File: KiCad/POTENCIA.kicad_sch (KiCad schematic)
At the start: 15 parts, among them J3 Conn_01x02_Pin, J7 Conn_01x02_Pin, J8 Conn_01x02_Pin, SW7 SW_SPST, U2 LM2596S-5, U3 L298N, U7 LM1117DT-3.3

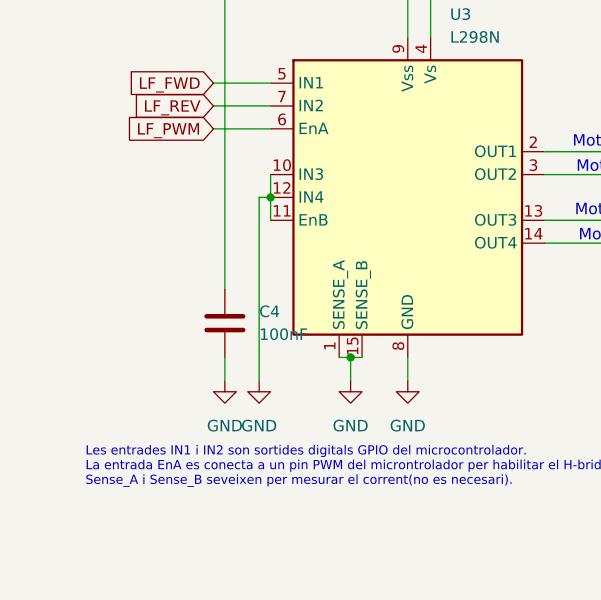
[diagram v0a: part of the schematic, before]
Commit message: aa
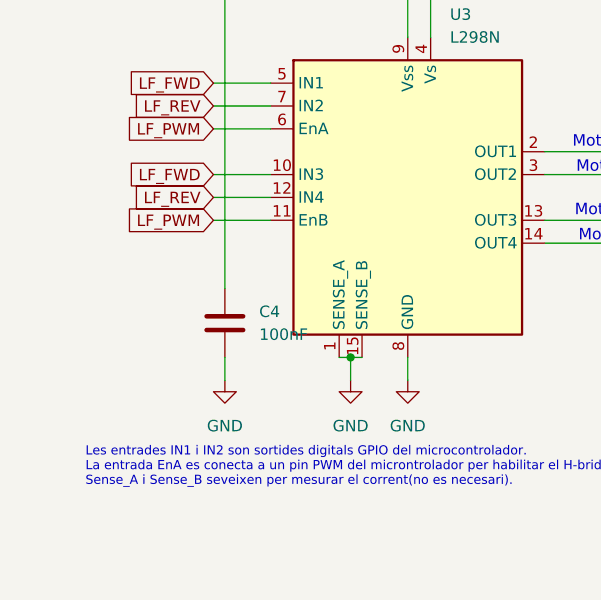
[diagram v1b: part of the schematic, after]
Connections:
- net GND: no longer U3.10 (IN3), U3.11 (EnB), U3.12 (IN4)
- net LF_FWD: now also U3.10 (IN3)
- net LF_PWM: now also U3.11 (EnB)
- net LF_REV: now also U3.12 (IN4)
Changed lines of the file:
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@@
-	)
-	(junction
-		(at 40.64 146.05)
-		(diameter 0)
-		(color 0 0 0 0)
 	)
 	(junction
@@
 	(wire
 		(pts
-			(xy 40.64 143.51) (xy 40.64 146.05)
-		)
-		(stroke
-			(width 0)
-			(type default)
-		)
-	)
-	(wire
-		(pts
 			(xy 177.8 58.42) (xy 184.15 58.42)
-		)
-		(stroke
-			(width 0)
-			(type default)
-		)
-	)
-	(wire
-		(pts
-			(xy 40.64 146.05) (xy 39.37 146.05)
 		)
 		(stroke
@@
 	(wire
 		(pts
+			(xy 34.29 143.51) (xy 40.64 143.51)
+		)
+		(stroke
+			(width 0)
+			(type default)
+		)
+	)
+	(wire
+		(pts
 			(xy 146.05 66.04) (xy 146.05 69.85)
 		)
@@
 	(wire
 		(pts
-			(xy 40.64 146.05) (xy 40.64 148.59)
-		)
-		(stroke
-			(width 0)
-			(type default)
-		)
-	)
-	(wire
-		(pts
 			(xy 130.81 58.42) (xy 133.35 58.42)
 		)
@@
 		(pts
 			(xy 133.35 58.42) (xy 135.89 58.42)
-		)
-		(stroke
-			(width 0)
-			(type default)
-		)
-	)
-	(wire
-		(pts
-			(xy 39.37 146.05) (xy 39.37 166.37)
 		)
 		(stroke
@@
 	(wire
 		(pts
+			(xy 34.29 146.05) (xy 40.64 146.05)
+		)
+		(stroke
+			(width 0)
+			(type default)
+		)
+	)
+	(wire
+		(pts
 			(xy 193.04 130.81) (xy 185.42 130.81)
+		)
+		(stroke
+			(width 0)
+			(type default)
+		)
+	)
+	(wire
+		(pts
+			(xy 34.29 148.59) (xy 40.64 148.59)
 		)
 		(stroke
@@
 		)
 	)
+	(global_label "LF_REV"
+		(shape input)
+		(at 34.29 146.05 180)
+		(fields_autoplaced yes)
+		(effects
+			(font
+				(size 1.27 1.27)
+			)
+			(justify right)
+		)
+		(property "Intersheetrefs" "${INTERSHEET_REFS}"
+			(at 24.7129 146.05 0)
+			(effects
+				(font
+					(size 1.27 1.27)
+				)
+				(justify right)
+				(hide yes)
+			)
+		)
+	)
 	(global_label "LF_FWD"
 		(shape input)
@@
 		)
 	)
+	(global_label "LF_FWD"
+		(shape input)
+		(at 34.29 143.51 180)
+		(fields_autoplaced yes)
+		(effects
+			(font
+				(size 1.27 1.27)
+			)
+			(justify right)
+		)
+		(property "Intersheetrefs" "${INTERSHEET_REFS}"
+			(at 24.4105 143.51 0)
+			(effects
+				(font
+					(size 1.27 1.27)
+				)
+				(justify right)
+				(hide yes)
+			)
+		)
+	)
 	(global_label "VCC"
 		(shape output)
@@
 				)
 				(justify left)
+				(hide yes)
+			)
+		)
+	)
+	(global_label "LF_PWM"
+		(shape input)
+		(at 34.29 148.59 180)
+		(fields_autoplaced yes)
+		(effects
+			(font
+				(size 1.27 1.27)
+			)
+			(justify right)
+		)
+		(property "Intersheetrefs" "${INTERSHEET_REFS}"
+			(at 24.0477 148.59 0)
+			(effects
+				(font
+					(size 1.27 1.27)
+				)
+				(justify right)
 				(hide yes)
 			)
@@
 					(unit 1)
 				)
-			)
-		)
-	)
-	(symbol
-		(lib_id "power:GND")
-		(at 39.37 166.37 0)
-		(unit 1)
-		(exclude_from_sim no)
-		(in_bom yes)
-		(on_board yes)
-		(dnp no)
-		(fields_autoplaced yes)
-		(property "Reference" "#PWR010"
-			(at 39.37 172.72 0)
-			(effects
-				(font
-					(size 1.27 1.27)
-				)
-				(hide yes)
-			)
-		)
-		(property "Value" "GND"
-			(at 39.37 171.45 0)
-			(effects
-				(font
-					(size 1.27 1.27)
-				)
-			)
-		)
-		(property "Footprint" ""
-			(at 39.37 166.37 0)
-			(effects
-				(font
-					(size 1.27 1.27)
-				)
-				(hide yes)
-			)
-		)
-		(property "Datasheet" ""
-			(at 39.37 166.37 0)
-			(effects
-				(font
-					(size 1.27 1.27)
-				)
-				(hide yes)
-			)
-		)
-		(property "Description" "Power symbol creates a global label with name \"GND\" , ground"
-			(at 39.37 166.37 0)
-			(effects
-				(font
-					(size 1.27 1.27)
-				)
-				(hide yes)
-			)
-		)
-		(pin "1"
-		)
-		(instances
-			(project "Grup_D_Llums"
-				(path "/88ef36bc-9439-47f2-adb5-e1da6bb8c9dd/c965bb79-4e48-4b35-b9c7-2e902c1fe9a5"
-					(reference "#PWR010")
-					(unit 1)
-				)

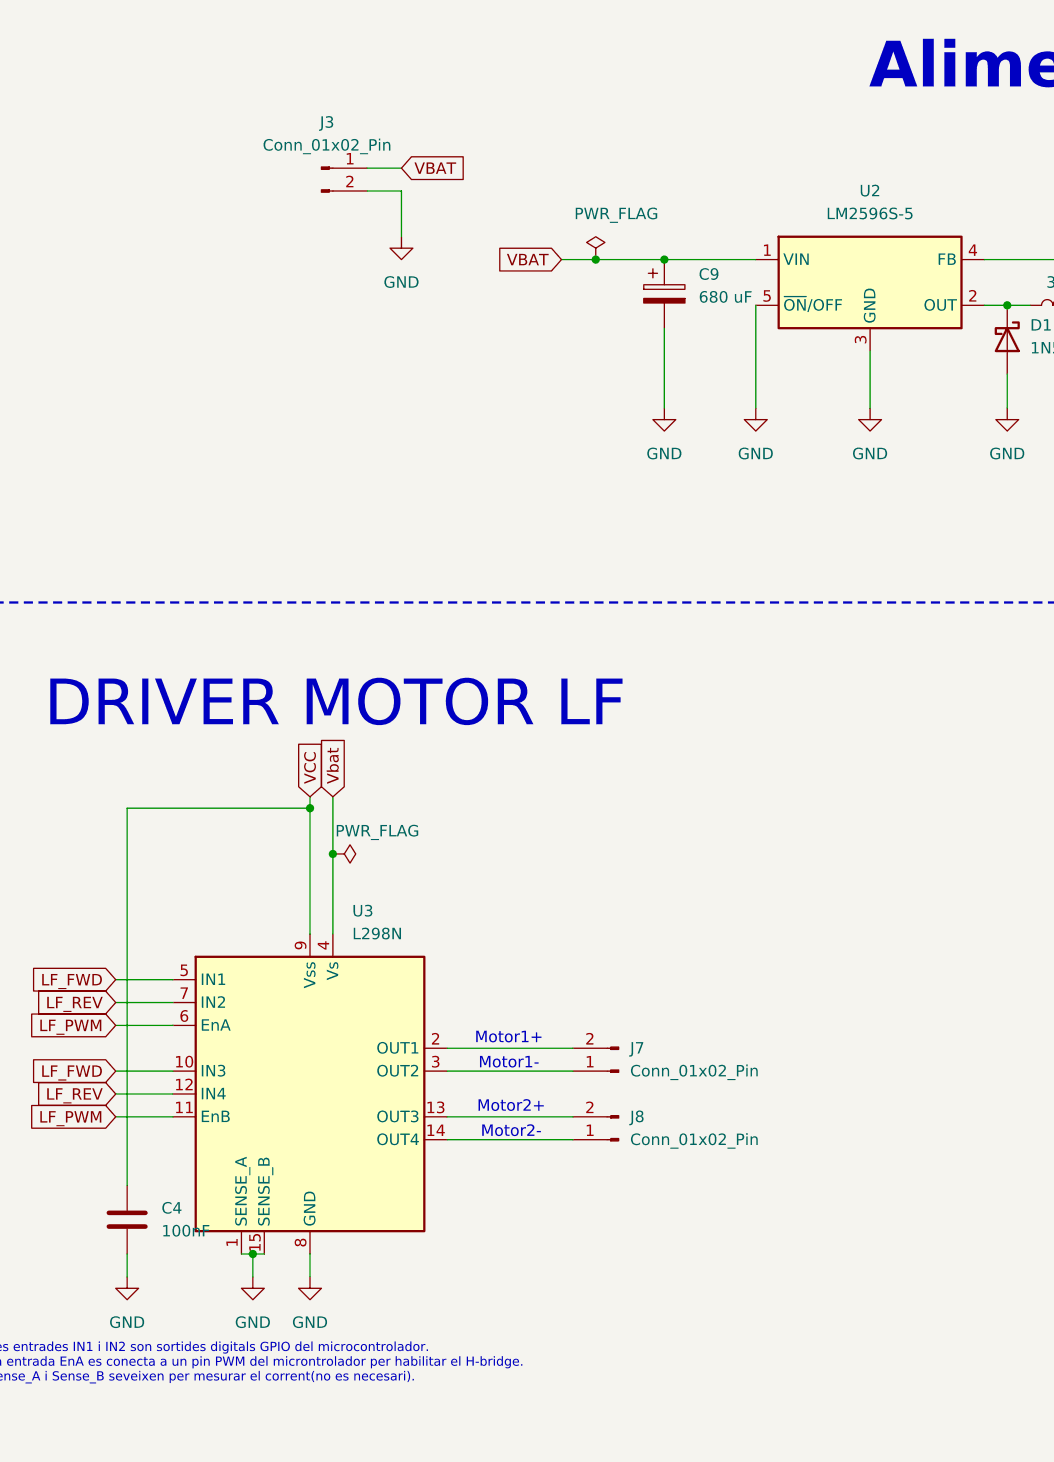
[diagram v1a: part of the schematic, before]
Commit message: Aa
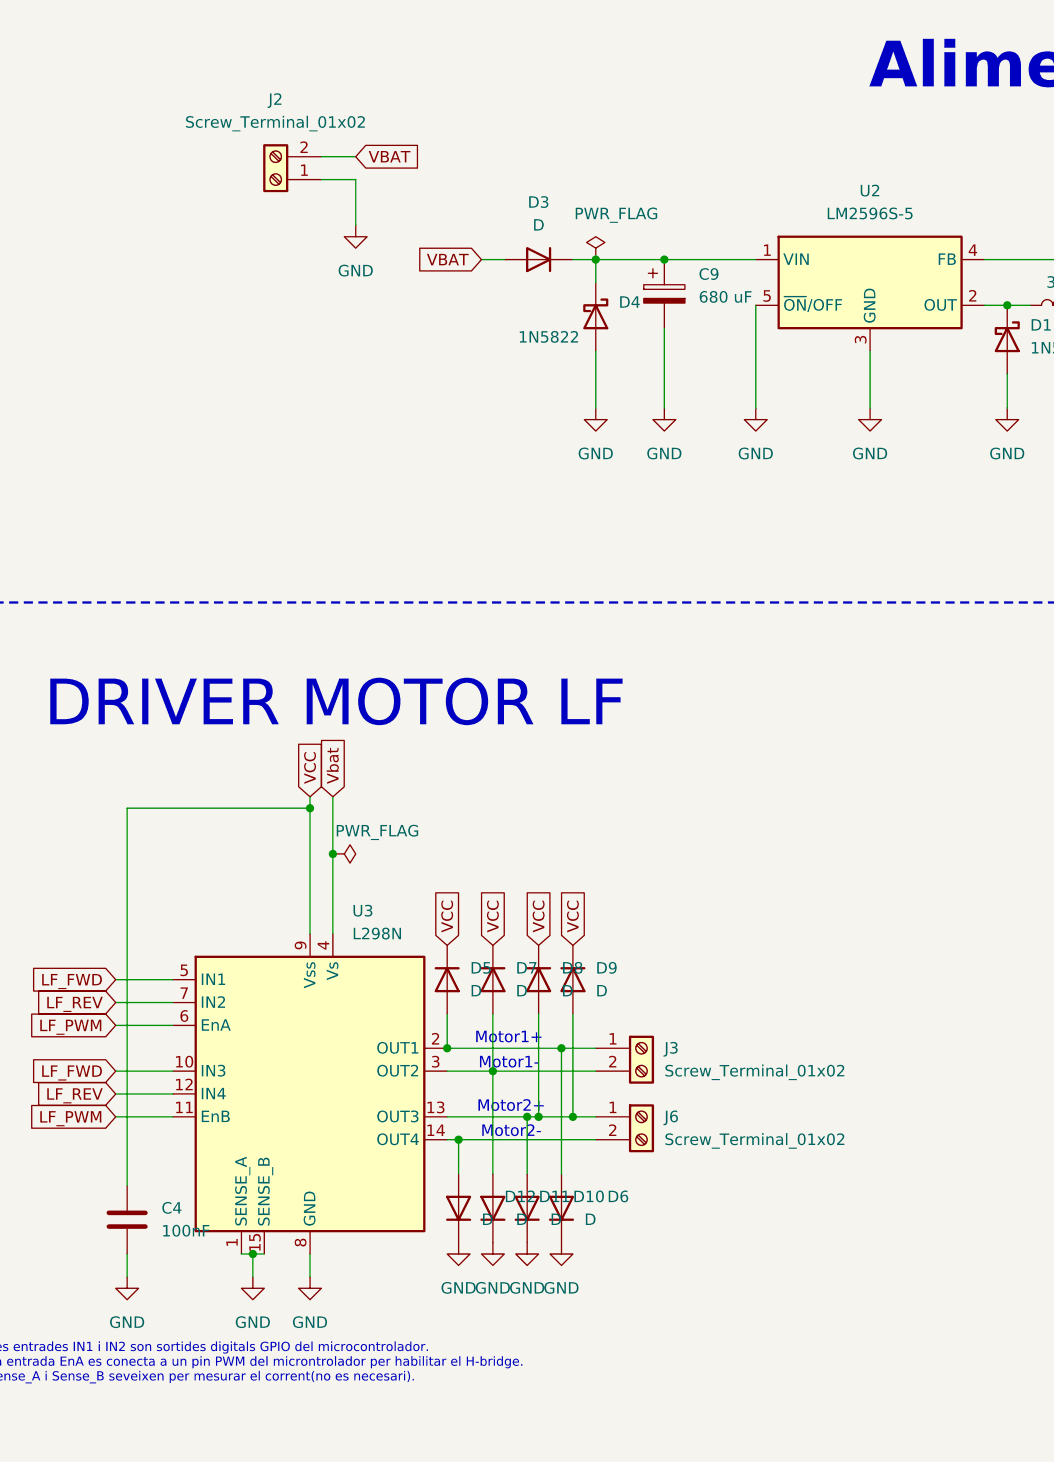
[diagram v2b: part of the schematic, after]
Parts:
- removed J3, J7, J8: Conn_01x02_Pin, symbol Connector:Conn_01x02_Pin
- added D10, D11, D12, D3, D5, D6, D7, D8, D9: D, symbol Device:D
- added D4: 1N5822, Diode_THT:D_DO-201AD_P15.24mm_Horizontal, symbol Diode:1N5822
- added J2, J3, J6: Screw_Terminal_01x02, symbol Connector:Screw_Terminal_01x02
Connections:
- net GND: now also D10.1 (K), D11.1 (K), D12.1 (K), D4.2 (A), D6.1 (K), J2.1 (Pin_1)
- net VBAT: now also D3.2 (A), J2.2 (Pin_2); no longer C9.1, U2.1 (VIN)
- net VCC: now also D5.1 (K), D7.1 (K), D8.1 (K), D9.1 (K)
- net at U3.3 (OUT2): now also D11.2 (A), D7.2 (A), J3.2 (Pin_2)
- net at U3.2 (OUT1): now also D5.2 (A), D6.2 (A), J3.1 (Pin_1)
- net at U3.14 (OUT4): now also D12.2 (A), J6.2 (Pin_2)
- net at U3.13 (OUT3): now also D10.2 (A), D8.2 (A), D9.2 (A), J6.1 (Pin_1)
- new net: C9.1, D3.1 (K), D4.1 (K), U2.1 (VIN)

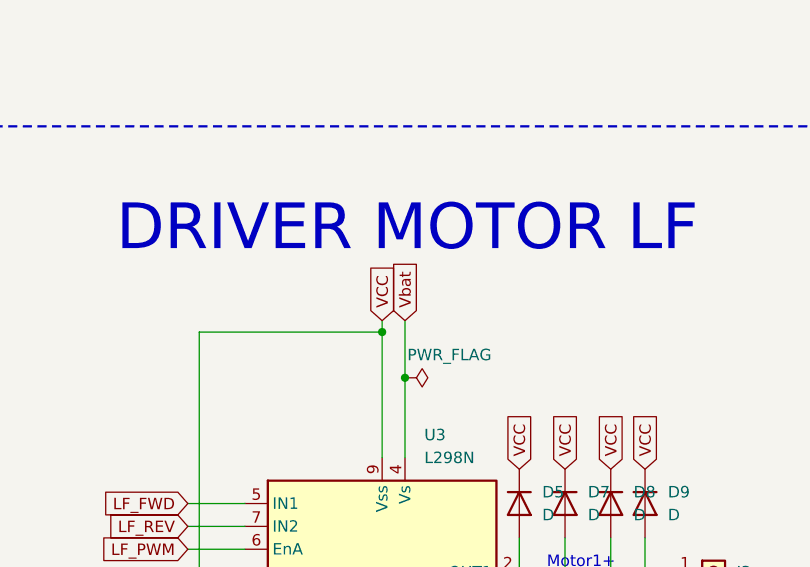
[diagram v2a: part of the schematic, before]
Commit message: Huellass
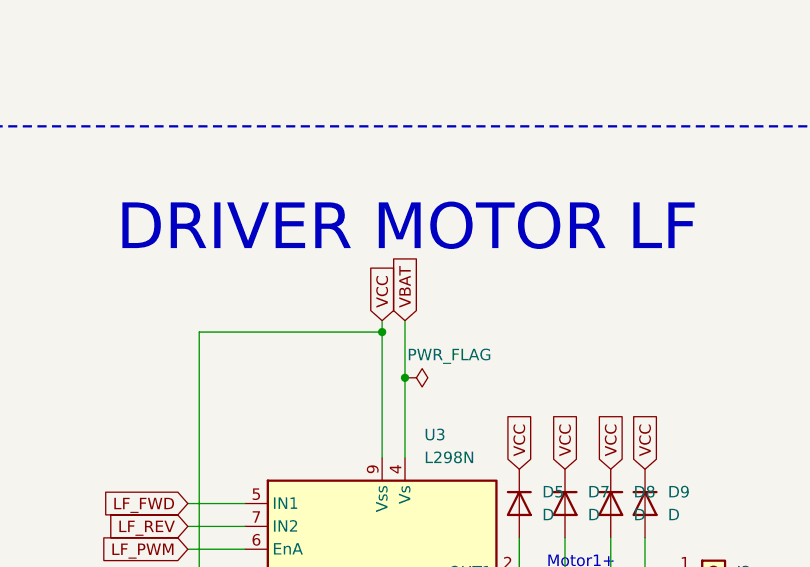
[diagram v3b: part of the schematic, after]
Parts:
- C1: footprint (none) -> Capacitor_THT:CP_Radial_D8.0mm_P3.50mm
- C10, C11, C4: footprint (none) -> Capacitor_SMD:C_0805_2012Metric
- C9: footprint (none) -> Capacitor_THT:CP_Radial_D10.0mm_P5.00mm
- D10, D11, D12, D3, D5, D6, D7, D8, D9: footprint (none) -> Diode_THT:D_DO-201AD_P15.24mm_Horizontal
- J2, J3, J6: footprint (none) -> TerminalBlock_Phoenix:TerminalBlock_Phoenix_MKDS-1,5-2-5.08_1x02_P5.08mm_Horizontal
- L1: footprint (none) -> Inductor_THT:L_Radial_D10.0mm_P5.00mm_Fastron_07M
- SW7: footprint (none) -> Button_Switch_THT:SW_PUSH_6mm
- pull_FC1: footprint (none) -> Resistor_SMD:R_0805_2012Metric
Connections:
- net Vbat is gone; now on net VBAT: U3.4 (Vs)
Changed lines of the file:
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@@
 		)
 	)
-	(global_label "Vbat"
+	(global_label "VBAT"
 		(shape input)
 		(at 58.42 113.03 90)
@@
 		)
 		(property "Intersheetrefs" "${INTERSHEET_REFS}"
-			(at 58.42 105.9325 90)
+			(at 58.42 105.63 90)
 			(effects
 				(font
@@
 			)
 		)
-		(property "Footprint" ""
+		(property "Footprint" "TerminalBlock_Phoenix:TerminalBlock_Phoenix_MKDS-1,5-2-5.08_1x02_P5.08mm_Horizontal"
 			(at 92.71 140.97 0)
 			(effects
@@
 			)
 		)
-		(property "Footprint" ""
+		(property "Footprint" "Diode_THT:D_DO-201AD_P15.24mm_Horizontal"
 			(at 81.28 53.34 0)
 			(effects
@@
 			)
 		)
-		(property "Footprint" ""
+		(property "Footprint" "Diode_THT:D_DO-201AD_P15.24mm_Horizontal"
 			(at 72.39 158.75 0)
 			(effects
@@
 			)
 		)
-		(property "Footprint" ""
+		(property "Footprint" "Diode_THT:D_DO-201AD_P15.24mm_Horizontal"
 			(at 83.82 158.75 0)
 			(effects
@@
 			)
 		)
-		(property "Footprint" ""
+		(property "Footprint" "Diode_THT:D_DO-201AD_P15.24mm_Horizontal"
 			(at 71.12 133.35 0)
 			(effects
@@
 			)
 		)
-		(property "Footprint" ""
+		(property "Footprint" "Button_Switch_THT:SW_PUSH_6mm"
 			(at 198.12 130.81 0)
 			(effects
@@
 			)
 		)
-		(property "Footprint" ""
+		(property "Footprint" "Inductor_THT:L_Radial_D10.0mm_P5.00mm_Fastron_07M"
 			(at 139.7 58.42 0)
 			(effects
@@
 			)
 		)
-		(property "Footprint" ""
+		(property "Footprint" "Diode_THT:D_DO-201AD_P15.24mm_Horizontal"
 			(at 76.2 133.35 0)
 			(effects
@@
 			)
 		)
-		(property "Footprint" ""
+		(property "Footprint" "Diode_THT:D_DO-201AD_P15.24mm_Horizontal"
 			(at 76.2 158.75 0)
 			(effects
@@
 			)
 		)
-		(property "Footprint" ""
+		(property "Footprint" "Capacitor_SMD:C_0805_2012Metric"
 			(at 184.15 62.23 0)
 			(effects
@@
 			)
 		)
-		(property "Footprint" ""
+		(property "Footprint" "TerminalBlock_Phoenix:TerminalBlock_Phoenix_MKDS-1,5-2-5.08_1x02_P5.08mm_Horizontal"
 			(at 52.07 44.45 0)
 			(effects
@@
 			)
 		)
-		(property "Footprint" ""
+		(property "Footprint" "Capacitor_SMD:C_0805_2012Metric"
 			(at 36.5252 163.83 0)
 			(effects
@@
 			)
 		)
-		(property "Footprint" ""
+		(property "Footprint" "TerminalBlock_Phoenix:TerminalBlock_Phoenix_MKDS-1,5-2-5.08_1x02_P5.08mm_Horizontal"
 			(at 92.71 148.59 0)
 			(effects
@@
 			)
 		)
-		(property "Footprint" ""
+		(property "Footprint" "Capacitor_THT:CP_Radial_D8.0mm_P3.50mm"
 			(at 147.0152 66.04 0)
 			(effects
@@
 			)
 		)
-		(property "Footprint" ""
+		(property "Footprint" "Resistor_SMD:R_0805_2012Metric"
 			(at 220.726 123.444 90)
 			(effects
@@
 			)
 		)
-		(property "Footprint" ""
+		(property "Footprint" "Diode_THT:D_DO-201AD_P15.24mm_Horizontal"
 			(at 85.09 133.35 0)
 			(effects
@@
 			)
 		)
-		(property "Footprint" ""
+		(property "Footprint" "Diode_THT:D_DO-201AD_P15.24mm_Horizontal"
 			(at 81.28 133.35 0)
 			(effects
@@
 			)
 		)
-		(property "Footprint" ""
+		(property "Footprint" "Diode_THT:D_DO-201AD_P15.24mm_Horizontal"
 			(at 80.01 158.75 0)
 			(effects
@@
 			)
 		)
-		(property "Footprint" ""
+		(property "Footprint" "Capacitor_THT:CP_Radial_D10.0mm_P5.00mm"
 			(at 96.2152 60.96 0)
 			(effects
@@
 			)
 		)
-		(property "Footprint" ""
+		(property "Footprint" "Capacitor_SMD:C_0805_2012Metric"
 			(at 153.67 62.23 0)
 			(effects
